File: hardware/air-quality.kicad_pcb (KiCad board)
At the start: 2 copper layers, 20 x 25 mm, 26 parts, among them P101 CON-SENSOR2, P102 DEBUG, P103 BOOT, U1 BME680, U103 DRILL, U104 DRILL, U105 DRILL, U106 DRILL, U2 XMC1404

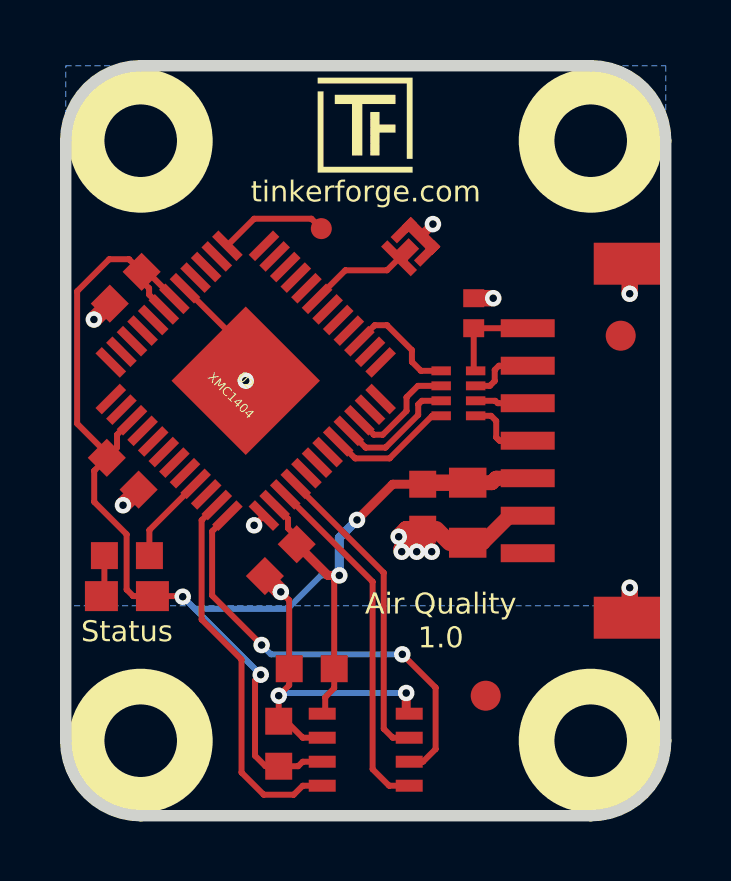
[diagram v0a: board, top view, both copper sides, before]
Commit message: update to new kicad version
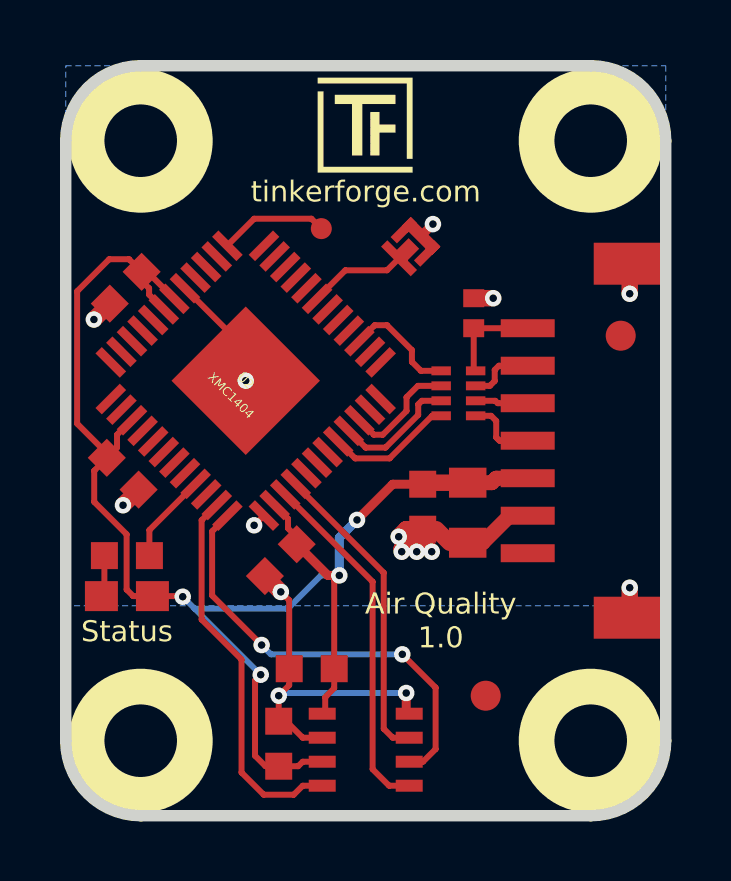
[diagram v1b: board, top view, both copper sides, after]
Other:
- net class Default removed
